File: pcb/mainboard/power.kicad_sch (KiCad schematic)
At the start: 30 parts

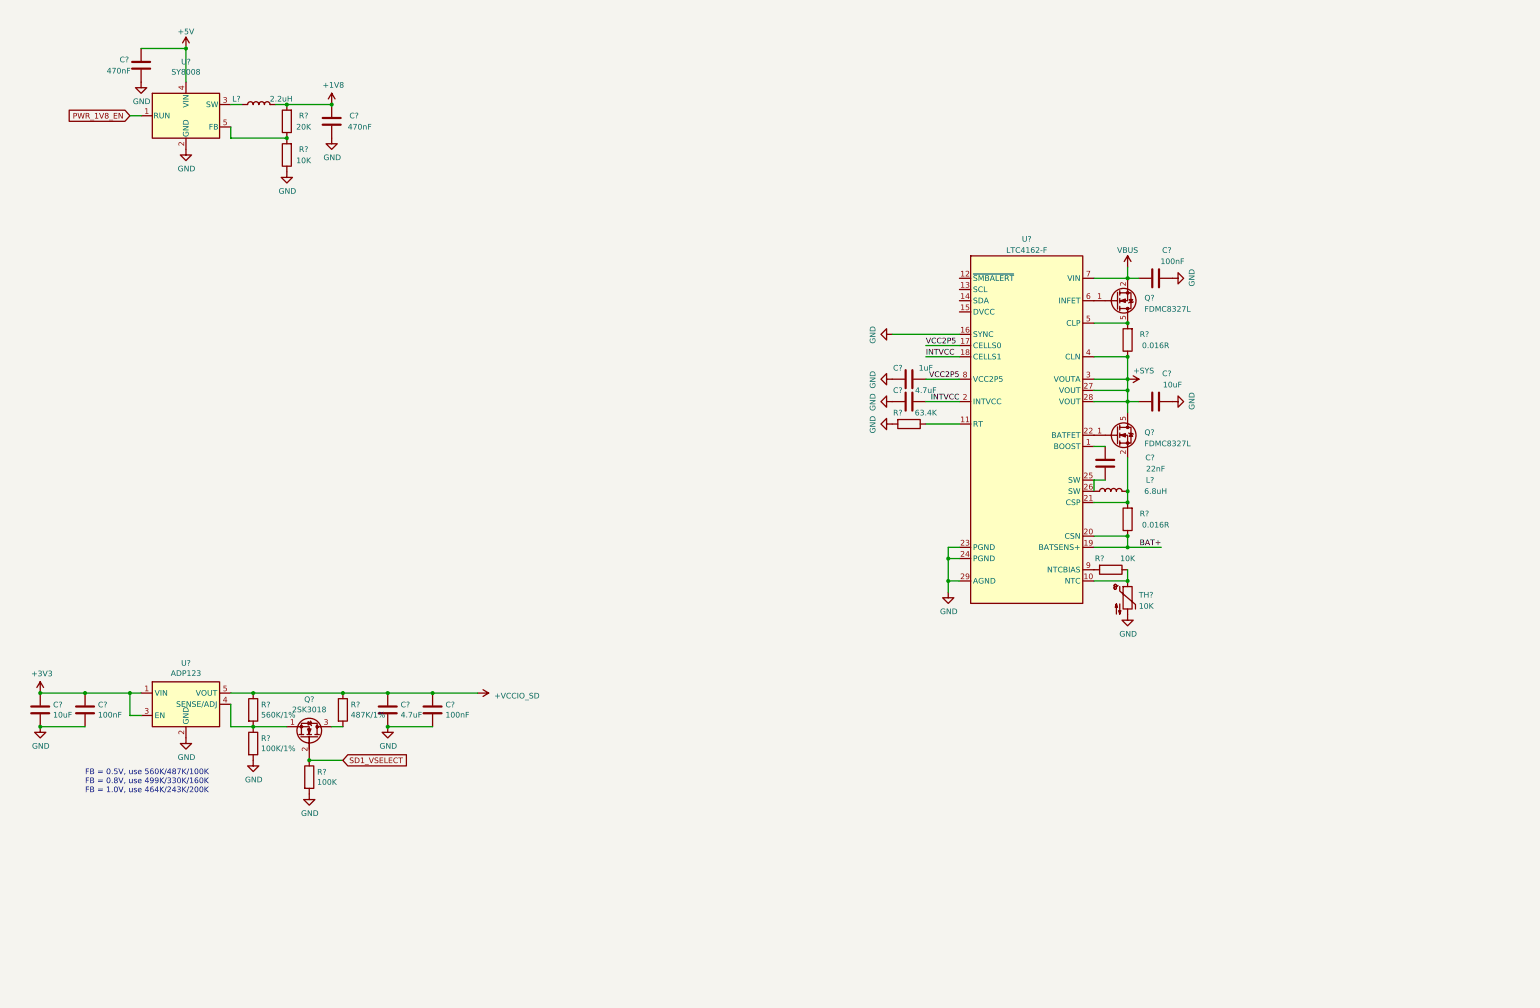
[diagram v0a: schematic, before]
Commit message: - pcb: r0p1 sch draft
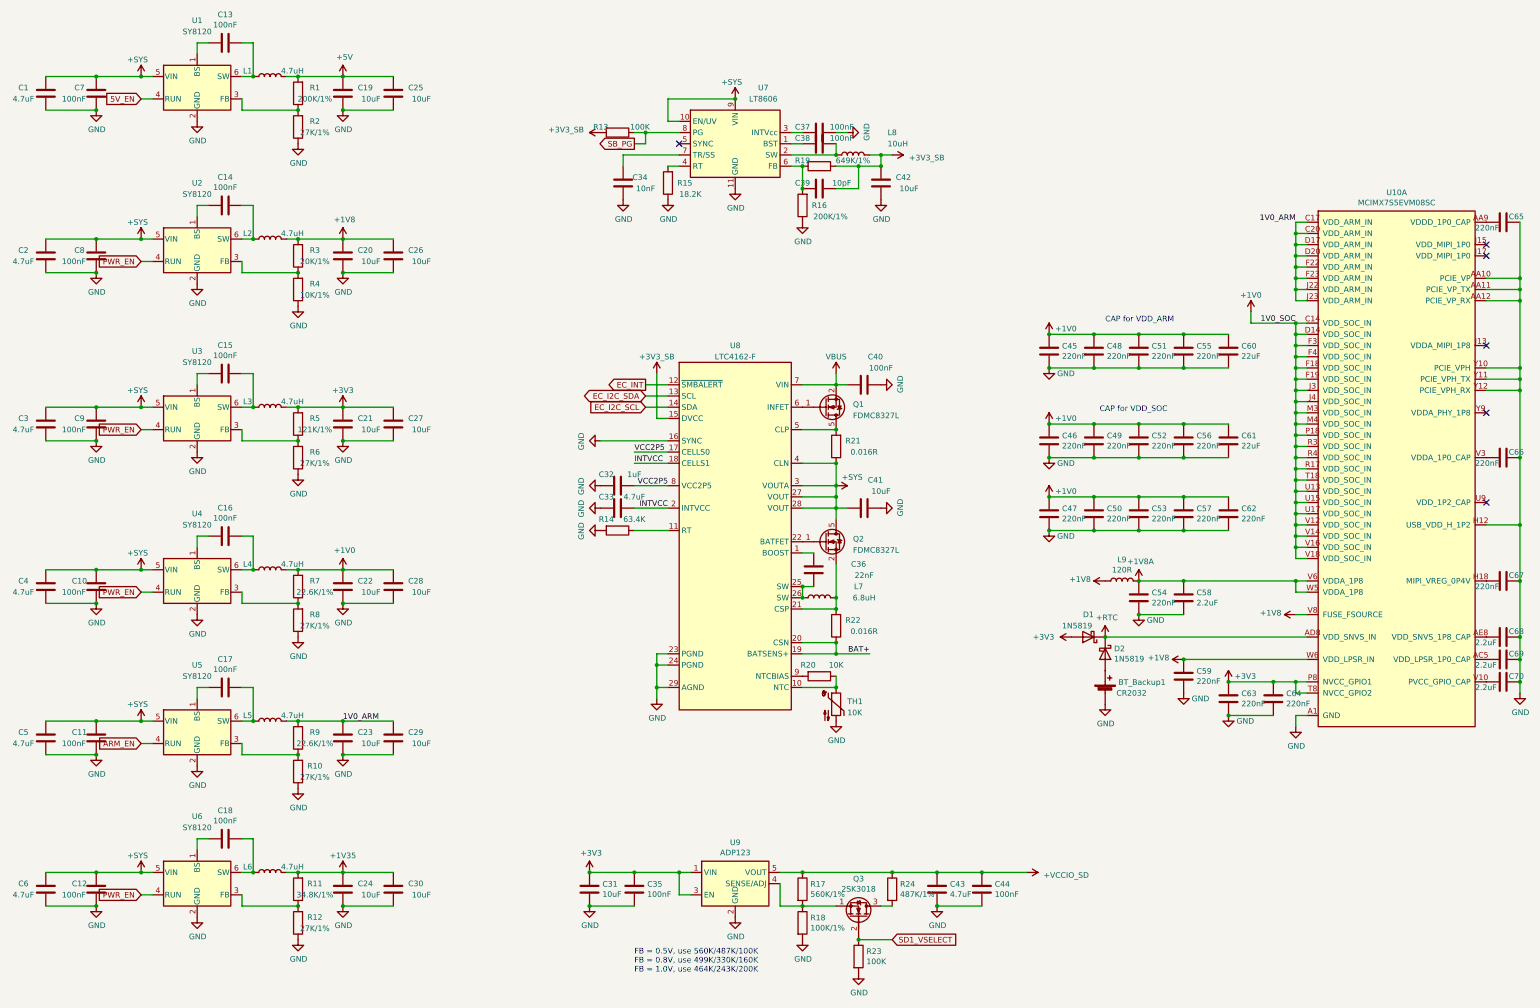
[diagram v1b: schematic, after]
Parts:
- removed C? (x2): 470nF, Capacitor_SMD:C_0402_1005Metric, symbol Device:C
- removed L?: 2.2uH, Inductor_SMD:L_Vishay_IHLP-1212, symbol Device:L
- removed R?: 10K, Resistor_SMD:R_0402_1005Metric, symbol Device:R
- removed R?: 20K, Resistor_SMD:R_0402_1005Metric, symbol Device:R
- removed U?: SY8008, Package_TO_SOT_SMD:TSOT-23-5, symbol symbols:SY8008
- added BT_Backup1: CR2032, footprints:BatteryHolder_CR1220, symbol Device:Battery_Cell
- added C1, C2, C3, C4, C5, C6: 4.7uF, Capacitor_SMD:C_0805_2012Metric, symbol Device:C
- added C10, C11, C12, C13, C14, C15, C16, C17, C18, C7, C8, C9: 100nF, Capacitor_SMD:C_0603_1608Metric, symbol Device:C
- added C19, C20, C21, C22, C23, C24: 10uF, Capacitor_SMD:C_0603_1608Metric, symbol Device:C
- added C25, C26, C27, C28, C29, C30, C42: 10uF, Capacitor_SMD:C_Elec_5x5.8, symbol Device:C
- added C34: 10nF, Capacitor_SMD:C_Elec_5x5.8, symbol Device:C
- added C37, C38: 100nF, Capacitor_SMD:C_0402_1005Metric, symbol Device:C
- added C39: 10pF, Capacitor_SMD:C_0402_1005Metric, symbol Device:C
- added C45, C46, C47, C48, C49, C50, C51, C52, C53, C54, C55, C56, C57, C59, C62, C63, C64, C65, C66, C67: 220nF, Capacitor_SMD:C_0402_1005Metric, symbol Device:C
- added C58, C68, C69, C70: 2.2uF, Capacitor_SMD:C_0402_1005Metric, symbol Device:C
- added C60, C61: 22uF, Capacitor_SMD:C_0603_1608Metric, symbol Device:C
- added D1, D2: 1N5819, Diode_SMD:D_SOD-123, symbol Device:D_Schottky
- added L1, L2, L3, L4, L5, L6: 4.7uH, Inductor_SMD:L_Vishay_IHLP-1212, symbol Device:L
- added L8: 10uH, symbol Device:L
- added L9: 120R, Inductor_SMD:L_0402_1005Metric, symbol Device:L
- added R1, R16: 200K/1%, Resistor_SMD:R_0603_1608Metric, symbol Device:R
- added R10, R12, R2, R6, R8: 27K/1%, Resistor_SMD:R_0603_1608Metric, symbol Device:R
- added R11: 34.8K/1%, Resistor_SMD:R_0603_1608Metric, symbol Device:R
- added R13: 100K, Resistor_SMD:R_0402_1005Metric, symbol Device:R
- added R15: 18.2K, Resistor_SMD:R_0603_1608Metric, symbol Device:R
- added R19: 649K/1%, Resistor_SMD:R_0402_1005Metric, symbol Device:R
- added R3: 20K/1%, Resistor_SMD:R_0603_1608Metric, symbol Device:R
- added R4: 10K/1%, Resistor_SMD:R_0603_1608Metric, symbol Device:R
- added R5: 121K/1%, Resistor_SMD:R_0603_1608Metric, symbol Device:R
- added R7, R9: 22.6K/1%, Resistor_SMD:R_0603_1608Metric, symbol Device:R
- added U1, U2, U3, U4, U5, U6: SY8120, Package_TO_SOT_SMD:TSOT-23-6, symbol symbols:SY8120
- added U10: MCIMX7S5EVM08SC, footprints:BGA-541_25x25_19.0x19.0mm, symbol symbols:MCIMX7S5EVM08SC
- added U7: LT8606, Package_SO:MSOP-10-1EP_3x3mm_P0.5mm_EP1.68x1.88mm_ThermalVias, symbol symbols:LT8606
- gave numbers to parts that had none: 24
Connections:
- net +1V8: now also C20.2, C26.2, C59.1, L2.2, L9.1, R3.2, U10.V8 (FUSE_FSOURCE), U10.W6 (VDD_LPSR_IN)
- net +3V3: now also C21.2, C27.2, C63.1, C64.1, D1.2 (A), L3.2, R5.2, U10.P8 (NVCC_GPIO1), U10.T8 (NVCC_GPIO2)
- net +5V: now also C19.2, C25.2, L1.2, R1.2
- net +SYS: now also C1.2, C10.2, C11.2, C12.2, C2.2, C3.2, C4.2, C5.2, C6.2, C7.2, C8.2, C9.2, U1.5 (VIN), U2.5 (VIN), U3.5 (VIN), U4.5 (VIN), U5.5 (VIN), U6.5 (VIN), U7.10 (EN/UV), U7.9 (VIN)
- net GND: now also BT_Backup1.2 (-), C1.1, C10.1, C11.1, C12.1, C19.1, C2.1, C20.1, C21.1, C22.1, C23.1, C24.1, C25.1, C26.1, C27.1, C28.1, C29.1, C3.1, C30.1, C34.1, C37.1, C4.1, C42.1, C45.2, C46.2, C47.2, C48.2, C49.2, C5.1, C50.2, C51.2, C52.2, C53.2, C54.2, C55.2, C56.2, C57.2, C58.2, C59.2, C6.1, C60.2, C61.2, C62.2, C63.2, C64.2, C65.1, C66.1, C67.1, C68.1, C69.1, C7.1, C70.1, C8.1, C9.1, R10.1, R12.1, R15.1, R16.1, R2.1, R4.1, R6.1, R8.1, U1.2 (GND), U10.A1 (GND), U10.A13 (GND), U10.A17 (GND), U10.A21 (GND), U10.A25 (GND), U10.A3 (GND), U10.A6 (GND), U10.A9 (GND), U10.AA1 (GND), U10.AA10 (PCIE_VP), U10.AA11 (PCIE_VP_TX), U10.AA12 (PCIE_VP_RX), U10.AA15 (GND), U10.AA2 (GND), U10.AA23 (GND), U10.AA6 (GND), U10.AA8 (GND), U10.AB12 (GND), U10.AB4 (GND), U10.AB5 (GND), U10.AB7 (GND), U10.AB9 (GND), U10.AC12 (GND), U10.AC15 (GND), U10.AC17 (GND), U10.AC19 (GND), U10.AC21 (GND), U10.AC23 (GND), U10.AC6 (GND), U10.AC9 (GND), U10.AD12 (GND), U10.AD2 (GND), U10.AD5 (GND), U10.AD7 (GND), U10.AD9 (GND), U10.AE1 (GND), U10.AE12 (GND), U10.AE24 (GND), U10.AE25 (GND), U10.AE5 (GND), U10.AE7 (GND), U10.AE9 (GND), U10.B13 (GND), U10.B17 (GND), U10.B21 (GND), U10.B3 (GND), U10.B6 (GND), U10.B9 (GND), U10.C13 (GND), U10.C15 (GND), U10.C16 (GND), U10.C18 (GND), U10.C19 (GND), U10.C9 (GND), U10.D1 (GND), U10.D10 (GND), U10.D2 (GND), U10.D22 (GND), U10.D4 (GND), U10.D7 (GND), U10.F11 (GND), U10.F13 (GND), U10.F7 (GND), U10.F8 (GND), U10.G11 (GND), U10.G13 (GND), U10.G15 (GND), U10.G17 (GND), U10.G19 (GND), U10.G22 (GND), U10.G4 (GND), U10.G7 (GND), U10.G9 (GND), U10.H1 (GND), U10.H12 (USB_VDD_H_1P2), U10.H2 (GND), U10.J19 (GND), U10.J7 (GND), U10.K10 (GND), U10.K12 (GND), U10.K14 (GND), U10.K16 (GND), U10.K22 (GND), U10.K4 (GND), U10.L11 (GND), U10.L13 (GND), U10.L15 (GND), U10.L19 (GND), U10.L7 (GND), U10.M10 (GND), U10.M12 (GND), U10.M14 (GND), U10.M16 (GND), U10.M24 (GND), U10.M25 (GND), U10.N11 (GND), U10.N13 (GND), U10.N15 (GND), U10.N19 (GND), U10.N4 (GND), U10.N7 (GND), U10.P10 (GND), U10.P12 (GND), U10.P14 (GND), U10.P16 (GND), U10.R11 (GND), U10.R13 (GND), U10.R15 (GND), U10.R19 (GND), U10.R20 (GND), U10.R21 (GND), U10.R23 (GND), U10.R7 (GND), U10.T10 (GND), U10.T12 (GND), U10.T14 (GND), U10.T16 (GND), U10.T20 (GND), U10.T4 (GND), U10.U11 (GND), U10.U19 (GND), U10.U20 (GND), U10.U23 (GND), U10.U7 (GND), U10.V20 (GND), U10.W1 (GND), U10.W11 (GND), U10.W13 (GND), U10.W15 (GND), U10.W17 (GND), U10.W19 (GND), U10.W2 (GND), U10.W20 (GND), U10.W23 (GND), U10.W4 (GND), U10.W7 (GND), U10.W9 (GND), U10.Y10 (PCIE_VPH), U10.Y11 (PCIE_VPH_TX), U10.Y12 (PCIE_VPH_RX), U10.Y13 (GND), U10.Y14 (GND), U10.Y15 (GND), U10.Y16 (GND), U10.Y17 (GND), U10.Y18 (GND), U10.Y19 (GND), U10.Y6 (GND), U2.2 (GND), U3.2 (GND), U4.2 (GND), U5.2 (GND), U6.2 (GND), U7.11 (GND)
- net EC_INT: now reaches U8.12 (~SMBALERT)
- net EC_I2C_SDA: now reaches U8.13 (SCL)
- net EC_I2C_SCL: now reaches U8.14 (SDA)
- net +3V3_SB: now reaches U8.15 (DVCC)
- net +3V3_SB: now also C39.1, C42.2, L8.2, R13.2, R19.1
- new net: C17.1, L5.1, U5.6 (SW)
- new net: R5.1, R6.2, U3.3 (FB)
- new net: C18.2, U6.1 (BS)
- new net: R11.1, R12.2, U6.3 (FB)
- new net: C18.1, L6.1, U6.6 (SW)
- new net: C14.1, L2.1, U2.6 (SW)
- new net: C15.1, L3.1, U3.6 (SW)
- new net: C39.2, R16.2, R19.2, U7.6 (FB)
- new net: R1.1, R2.2, U1.3 (FB)
- new net: BT_Backup1.1 (+), D2.2 (A)
- new net: R7.1, R8.2, U4.3 (FB)
- new net: C69.2, U10.AC5 (VDD_LPSR_1P0_CAP)
- new net: C15.2, U3.1 (BS)
- new net: C17.2, U5.1 (BS)
- new net: R10.2, R9.1, U5.3 (FB)
- new net: C13.1, L1.1, U1.6 (SW)
- new net: C16.2, U4.1 (BS)
- new net: C16.1, L4.1, U4.6 (SW)
- new net: R15.2, U7.4 (RT)
- new net: C34.2, U7.7 (TR/SS)
- new net: C66.2, U10.V3 (VDDA_1P0_CAP)
- new net: C14.2, U2.1 (BS)
- new net: C65.2, U10.AA9 (VDDD_1P0_CAP)
- new net: C68.2, U10.AE8 (VDD_SNVS_1P8_CAP)
- new net: C67.2, U10.H18 (MIPI_VREG_0P4V)
- new net: C70.2, U10.V10 (PVCC_GPIO_CAP)
- new net: C38.1, L8.1, U7.2 (SW)
- new net: C38.2, U7.1 (BST)
- new net: R3.1, R4.2, U2.3 (FB)
- new net: C13.2, U1.1 (BS)
- new net: C37.2, U7.3 (INTVcc)
- new net +1V0: C22.2, C28.2, C45.1, C46.1, C47.1, C48.1, C49.1, C50.1, C51.1, C52.1, C53.1, C55.1, C56.1, C57.1, C60.1, C61.1, C62.1, L4.2, R7.2, U10.C14 (VDD_SOC_IN), U10.D14 (VDD_SOC_IN), U10.F18 (VDD_SOC_IN), U10.F19 (VDD_SOC_IN), U10.F3 (VDD_SOC_IN), U10.F4 (VDD_SOC_IN), U10.J3 (VDD_SOC_IN), U10.J4 (VDD_SOC_IN), U10.M3 (VDD_SOC_IN), U10.M4 (VDD_SOC_IN), U10.P18 (VDD_SOC_IN), U10.R17 (VDD_SOC_IN), U10.R3 (VDD_SOC_IN), U10.R4 (VDD_SOC_IN), U10.T18 (VDD_SOC_IN), U10.U13 (VDD_SOC_IN), U10.U15 (VDD_SOC_IN), U10.U17 (VDD_SOC_IN), U10.V12 (VDD_SOC_IN), U10.V14 (VDD_SOC_IN), U10.V16 (VDD_SOC_IN), U10.V18 (VDD_SOC_IN)
- new net +1V35: C24.2, C30.2, L6.2, R11.2
- new net +1V8A: C54.1, C58.1, L9.2, U10.V6 (VDDA_1P8), U10.W5 (VDDA_1P8)
- new net +RTC: D1.1 (K), D2.1 (K), U10.AD8 (VDD_SNVS_IN)
- new net 1V0_ARM: C23.2, C29.2, L5.2, R9.2, U10.C17 (VDD_ARM_IN), U10.C20 (VDD_ARM_IN), U10.D17 (VDD_ARM_IN), U10.D20 (VDD_ARM_IN), U10.F22 (VDD_ARM_IN), U10.F23 (VDD_ARM_IN), U10.J22 (VDD_ARM_IN), U10.J23 (VDD_ARM_IN)
- new net 5V_EN: U1.4 (RUN)
- new net ARM_EN: U5.4 (RUN)
- new net PWR_EN: U2.4 (RUN), U3.4 (RUN), U4.4 (RUN), U6.4 (RUN)
- new net SB_PG: R13.1, U7.8 (PG)
- no-connect marks 0 -> 6
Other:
- note added: "CAP for VDD_ARM"
- note added: "CAP for VDD_SOC"
- moved on the sheet: C31, C32, C33, C35, C36, C40, C41, C43, C44, L7, Q1, Q2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
